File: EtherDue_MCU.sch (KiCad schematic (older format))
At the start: 29 parts, among them IC201 ATSAM3X8E, SW201 ERASE, SW202 RESET, U202 FDN340P, U203 LMV358IDGKR, X201 TXC 7A 12MHz 18pF, X202 ABS07L 32.768kHz

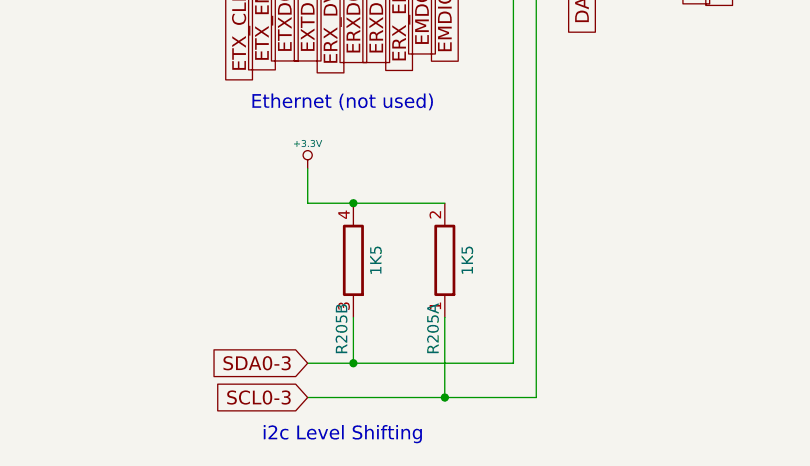
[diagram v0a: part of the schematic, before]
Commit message: Tweak schematics, netlist
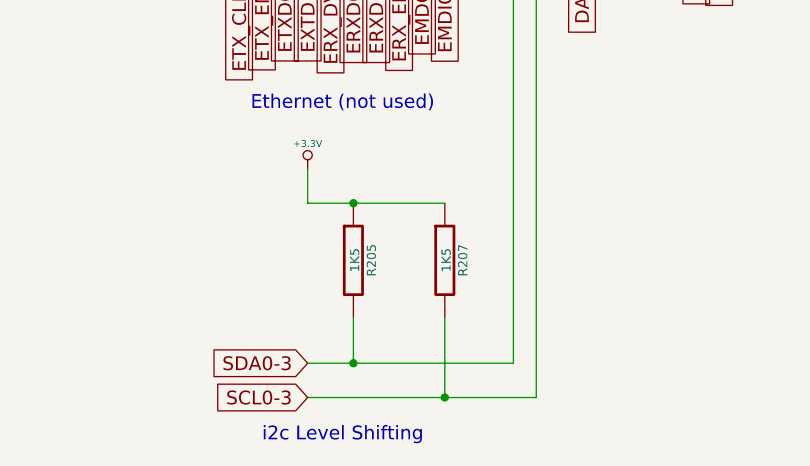
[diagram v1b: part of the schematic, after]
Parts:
- removed R205: 1K5, symbol RES_PACK4_IND
- added R205, R207: 1K5, ~, symbol R
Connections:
- net +3.3V: now also R205.1, R207.1
- net SCL0-3: now also R207.2
- net SDA0-3: now also R205.2
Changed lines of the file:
@@
-EESchema Schematic File Version 2  date Thu 06 Jun 2013 15:43:54 EST
+EESchema Schematic File Version 2  date Thu 06 Jun 2013 17:31:40 EST
 LIBS:freetronics_kicad_sch_lib
 LIBS:power
@@
 	1    6700 9750
 	1    0    0    -1
-$EndComp
-$Comp
-L RES_PACK4_IND R205
-U 1 1 5163C001
-P 7300 10150
-F 0 "R205" H 7000 10200 50  0000 C CNN
-F 1 "1K5" H 7300 10050 50  0000 C CNN
-F 2 "" H 7300 10150 60  0001 C CNN
-F 3 "" H 7300 10150 60  0001 C CNN
-	1    7300 10150
-	0    -1   -1   0
-$EndComp
-$Comp
-L RES_PACK4_IND R205
-U 2 1 5163BFF9
-P 6900 10150
-F 0 "R205" H 6600 10200 50  0000 C CNN
-F 1 "1K5" H 6900 10050 50  0000 C CNN
-F 2 "" H 6900 10150 60  0001 C CNN
-F 3 "" H 6900 10150 60  0001 C CNN
-	2    6900 10150
-	0    -1   -1   0
 $EndComp
 NoConn ~ 8700 8450
@@
 	1    0    0    -1
 $EndComp
+$Comp
+L R R205
+U 1 1 51B04B7A
+P 6900 10150
+F 0 "R205" V 6980 10150 40  0000 C CNN
+F 1 "1K5" V 6907 10151 40  0000 C CNN
+F 2 "~" V 6830 10150 30  0000 C CNN
+F 3 "~" H 6900 10150 30  0000 C CNN
+	1    6900 10150
+	1    0    0    -1
+$EndComp
+$Comp
+L R R207
+U 1 1 51B04B8E
+P 7300 10150
+F 0 "R207" V 7380 10150 40  0000 C CNN
+F 1 "1K5" V 7307 10151 40  0000 C CNN
+F 2 "~" V 7230 10150 30  0000 C CNN
+F 3 "~" H 7300 10150 30  0000 C CNN
+	1    7300 10150
+	1    0    0    -1
+$EndComp
